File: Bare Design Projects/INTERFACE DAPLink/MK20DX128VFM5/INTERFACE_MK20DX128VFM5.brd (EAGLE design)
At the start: 26 parts, among them CON1 47346-0001, CON2 TC2050-IDC-NL, U2 TLV1117LV33DCYR, U3 IF_MK20DX128VFM5, Y1 CSTCE8M00G55-R0

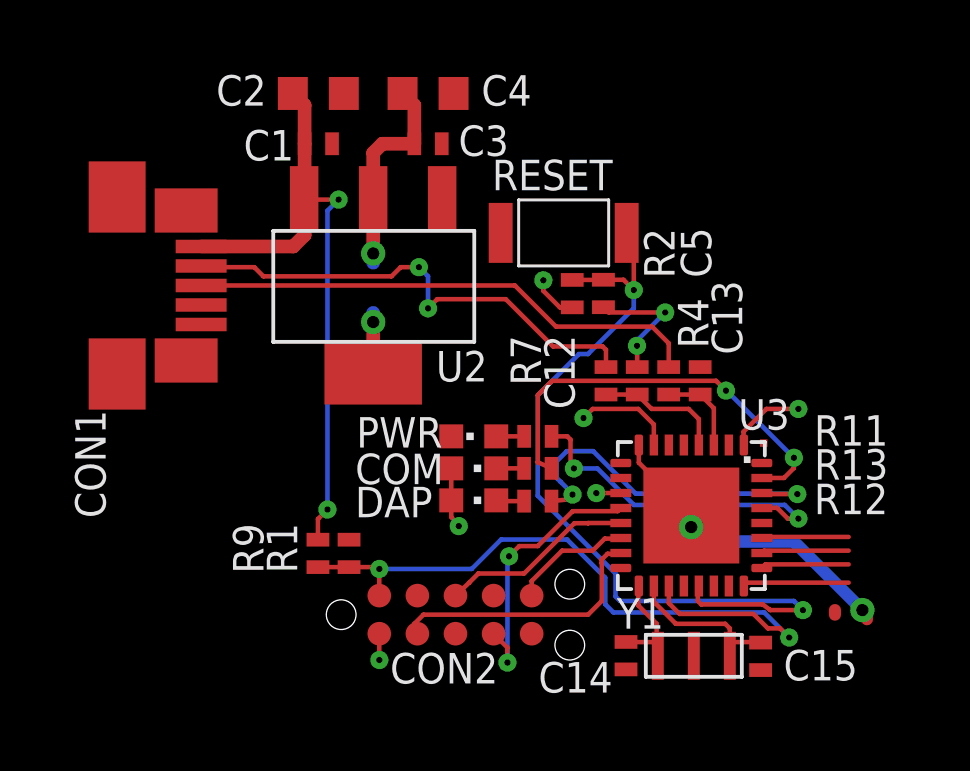
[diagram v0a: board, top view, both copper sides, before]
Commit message: Fixed PDF and name errors
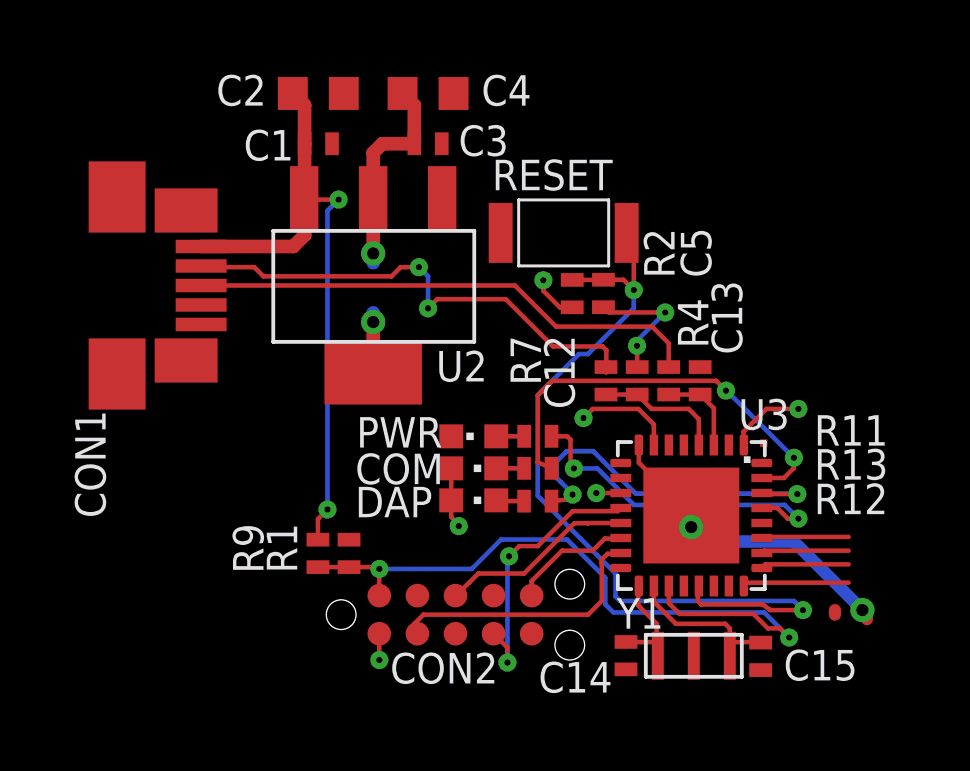
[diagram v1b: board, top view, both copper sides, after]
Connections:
- net DAP_NRESET renamed TGT_NRESET
- net DAP_RX renamed TGT_RX
- net DAP_SWCLK renamed TGT_SWCLK
- net DAP_SWDIO renamed TGT_SWDIO
- net DAP_TX renamed TGT_TX
- net DAP_USB_D+ renamed TGT_USB_D+
- net DAP_USB_D- renamed TGT_USB_D-
- net TCLK renamed IF_SWCLK
- net TDI renamed IF_TDI
- net TDO renamed IF_TDO
- net TMS renamed IF_SWDIO
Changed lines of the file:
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@@
 <wire x1="11.8872" y1="-5.9436" x2="12.0396" y2="-6.096" width="0.4064" layer="1"/>
 <wire x1="12.0396" y1="-6.096" x2="12.0396" y2="-6.2484" width="0.4064" layer="1"/>
+<wire x1="-2.1336" y1="9.6012" x2="-1.7408" y2="11.2776" width="0" layer="19" extent="1-1"/>
+<wire x1="-2.1196" y1="7.7812" x2="-2.1336" y2="9.6012" width="0" layer="19" extent="1-1"/>
+<wire x1="-0.1696" y1="6.6294" x2="-2.1196" y2="7.7812" width="0" layer="19" extent="1-1"/>
+<wire x1="-5.3984" y1="11.2776" x2="-1.7408" y2="11.2776" width="0" layer="19" extent="1-1"/>
+<wire x1="-5.7912" y1="9.6012" x2="-5.3984" y2="11.2776" width="0" layer="19" extent="1-1"/>
+<wire x1="3.25628125" y1="4.1529" x2="-0.1696" y2="6.6294" width="0" layer="19" extent="1-1"/>
+<wire x1="6.479540625" y1="2.156459375" x2="5.52958125" y2="3.977640625" width="0" layer="19" extent="1-1"/>
+<wire x1="4.4349" y1="-0.441459375" x2="4.3815" y2="2.156459375" width="0" layer="19" extent="1-1"/>
+<wire x1="6.17981875" y1="-3.177540625" x2="6.1849" y2="-2.791459375" width="0" layer="19" extent="1-1"/>
+<wire x1="10.9728" y1="-5.9436" x2="11.8872" y2="-5.9436" width="0" layer="19" extent="1-1"/>
+<wire x1="7.4349" y1="-0.441459375" x2="6.1849" y2="-2.791459375" width="0" layer="19" extent="1-1"/>
+<wire x1="8.493759375" y1="-7.942578125" x2="10.9728" y2="-6.096" width="0" layer="19" extent="1-1"/>
+<wire x1="6.2676" y1="-7.4676" x2="8.493759375" y2="-7.942578125" width="0" layer="19" extent="1-1"/>
+<wire x1="4.00811875" y1="-7.91971875" x2="6.2676" y2="-7.4676" width="0" layer="19" extent="1-1"/>
+<wire x1="0.8636" y1="-6.731" x2="4.00811875" y2="-7.91971875" width="0" layer="19" extent="1-1"/>
+<wire x1="-1.6764" y1="-6.731" x2="0.8636" y2="-6.731" width="0" layer="19" extent="1-1"/>
+<wire x1="-5.224778125" y1="-3.596640625" x2="-1.6764" y2="-6.731" width="0" layer="19" extent="1-1"/>
+<wire x1="-1.8168" y1="-0.1524" x2="-5.224778125" y2="-3.596640625" width="0" layer="19" extent="1-1"/>
+<wire x1="-10.154" y1="3.5768" x2="-5.7912" y2="9.6012" width="0" layer="19" extent="1-1"/>
 </signal>
 <signal name="IF_NRESET">
@@
 <wire x1="4.00811875" y1="-7.00531875" x2="4.0132" y2="-7.0104" width="0.1524" layer="1"/>
 <wire x1="4.0132" y1="-7.0104" x2="5.0292" y2="-7.0104" width="0.1524" layer="1"/>
-</signal>
-<signal name="DAP_USB_D-">
-<contactref element="R7" pad="1"/>
-<wire x1="3.3401" y1="2.156459375" x2="3.3401" y2="2.733040625" width="0.1524" layer="1"/>
-<wire x1="3.3401" y1="2.733040625" x2="3.228340625" y2="2.8448" width="0.1524" layer="1"/>
-<wire x1="3.228340625" y1="2.8448" x2="1.5748" y2="2.8448" width="0.1524" layer="1"/>
-<contactref element="CON1" pad="D-"/>
-<wire x1="1.5748" y1="2.8448" x2="0" y2="4.4196" width="0.1524" layer="1"/>
-<wire x1="0" y1="4.4196" x2="-2.286" y2="4.4196" width="0.1524" layer="1"/>
-<wire x1="-2.286" y1="4.4196" x2="-2.5908" y2="4.1148" width="0.1524" layer="1"/>
-<via x="-2.5908" y="4.1148" extent="1-16" drill="0.2032"/>
-<wire x1="-2.5908" y1="4.1148" x2="-2.5908" y2="5.1816" width="0.1524" layer="16"/>
-<wire x1="-2.5908" y1="5.1816" x2="-2.8956" y2="5.4864" width="0.1524" layer="16"/>
-<via x="-2.8956" y="5.4864" extent="1-16" drill="0.2032"/>
-<wire x1="-2.8956" y1="5.4864" x2="-3.5052" y2="5.4864" width="0.1524" layer="1"/>
-<wire x1="-3.5052" y1="5.4864" x2="-3.81" y2="5.1816" width="0.1524" layer="1"/>
-<wire x1="-3.81" y1="5.1816" x2="-8.0772" y2="5.1816" width="0.1524" layer="1"/>
-<wire x1="-8.0772" y1="5.1816" x2="-8.382" y2="5.4864" width="0.1524" layer="1"/>
-<wire x1="-8.382" y1="5.4864" x2="-10.1136" y2="5.4864" width="0.1524" layer="1"/>
-<wire x1="-10.1136" y1="5.4864" x2="-10.154" y2="5.5268" width="0.1524" layer="1"/>
-</signal>
-<signal name="DAP_USB_D+">
-<contactref element="R4" pad="1"/>
-<wire x1="5.43051875" y1="2.156459375" x2="5.43051875" y2="2.95148125" width="0.1524" layer="1"/>
-<wire x1="5.43051875" y1="2.95148125" x2="4.8768" y2="3.5052" width="0.1524" layer="1"/>
-<wire x1="4.8768" y1="3.5052" x2="1.6764" y2="3.5052" width="0.1524" layer="1"/>
-<contactref element="CON1" pad="D+"/>
-<wire x1="-10.154" y1="4.8768" x2="0.3048" y2="4.8768" width="0.1524" layer="1"/>
-<wire x1="0.3048" y1="4.8768" x2="1.6764" y2="3.5052" width="0.1524" layer="1"/>
 </signal>
 <signal name="+3.3V">
@@
 <via x="9.7536" y="0.762" extent="1-16" drill="0.2032"/>
 <wire x1="9.7536" y1="0.762" x2="9.906" y2="0.762" width="0.1524" layer="16"/>
-</signal>
-<signal name="DAP_NRESET">
+<wire x1="-1.56718125" y1="-3.14451875" x2="-4.2164" y2="-6.731" width="0" layer="19" extent="1-16"/>
+<wire x1="-4.4196" y1="1.9812" x2="-1.8168" y2="-1.2192" width="0" layer="19" extent="1-1"/>
+<wire x1="-4.4196" y1="5.6388" x2="-4.4196" y2="3.9624" width="0" layer="19" extent="16-16"/>
+<wire x1="3.037840625" y1="-2.17678125" x2="-1.49098125" y2="-3.14198125" width="0" layer="19" extent="16-16"/>
+<wire x1="4.9349" y1="-0.441459375" x2="3.8349" y2="-2.041459375" width="0" layer="19" extent="1-1"/>
+<wire x1="7.9248" y1="-0.431359375" x2="4.9349" y2="-0.441459375" width="0" layer="19" extent="1-1"/>
+<wire x1="2.21488125" y1="4.14781875" x2="2.8956" y2="0.762" width="0" layer="19" extent="1-1"/>
+</signal>
+<signal name="TGT_NRESET">
 <contactref element="RESET" pad="P$2"/>
 <wire x1="4.0304" y1="6.6294" x2="4.2672" y2="6.3246" width="0.1524" layer="1"/>
@@
 <wire x1="9.906" y1="-5.9436" x2="9.6012" y2="-5.6388" width="0.1524" layer="16"/>
 </signal>
-<signal name="DAP_TX">
+<signal name="TGT_TX">
 <contactref element="U3" pad="24"/>
 <wire x1="7.9349" y1="-5.141459375" x2="8.047159375" y2="-5.0292" width="0.1524" layer="1"/>
@@
 <wire x1="-6.67778125" y1="7.73938125" x2="-6.7196" y2="7.7812" width="0.1524" layer="1"/>
 </signal>
-<signal name="TMS">
+<signal name="IF_SWDIO">
 <contactref element="U3" pad="15"/>
 <contactref element="CON2" pad="2"/>
@@
 <wire x1="3.80981875" y1="-4.066540625" x2="3.8349" y2="-4.041459375" width="0.1524" layer="1"/>
 </signal>
-<signal name="TDO">
+<signal name="IF_TDO">
 <contactref element="U3" pad="14"/>
 <contactref element="CON2" pad="6"/>
@@
 <wire x1="3.815278125" y1="-3.56108125" x2="3.8349" y2="-3.541459375" width="0.1524" layer="1"/>
 </signal>
-<signal name="TDI">
+<signal name="IF_TDI">
 <contactref element="U3" pad="13"/>
 <contactref element="CON2" pad="8"/>
@@
 <wire x1="2.7432" y1="-3.048" x2="2.749740625" y2="-3.041459375" width="0.1524" layer="1"/>
 </signal>
-<signal name="TCLK">
+<signal name="IF_SWCLK">
 <contactref element="U3" pad="12"/>
 <contactref element="CON2" pad="4"/>
@@
 <wire x1="-0.3168" y1="-0.1524" x2="0.612140625" y2="-0.1524" width="0.1524" layer="1"/>
 </signal>
-<signal name="DAP_SWCLK">
+<signal name="TGT_SWCLK">
 <contactref element="U3" pad="26"/>
 <wire x1="8.5349" y1="-4.041459375" x2="8.613959375" y2="-3.9624" width="0.1524" layer="1"/>
 <wire x1="8.613959375" y1="-3.9624" x2="11.43" y2="-3.9624" width="0.1524" layer="1"/>
 </signal>
-<signal name="DAP_SWDIO">
+<signal name="TGT_SWDIO">
 <contactref element="U3" pad="27"/>
 <wire x1="8.5349" y1="-3.541459375" x2="8.571159375" y2="-3.5052" width="0.1524" layer="1"/>
 <wire x1="8.571159375" y1="-3.5052" x2="11.43" y2="-3.5052" width="0.1524" layer="1"/>
 </signal>
-<signal name="DAP_RX">
+<signal name="TGT_RX">
 <contactref element="U3" pad="25"/>
 <wire x1="8.5349" y1="-4.541459375" x2="8.656759375" y2="-4.4196" width="0.1524" layer="1"/>
 <wire x1="8.656759375" y1="-4.4196" x2="11.43" y2="-4.4196" width="0.1524" layer="1"/>
 </signal>
+<signal name="TGT_USB_D+">
+<contactref element="R4" pad="1"/>
+<wire x1="5.43051875" y1="2.95148125" x2="4.8768" y2="3.5052" width="0.1524" layer="1"/>
+<wire x1="4.8768" y1="3.5052" x2="1.6764" y2="3.5052" width="0.1524" layer="1"/>
+<contactref element="CON1" pad="D+"/>
+<wire x1="-10.154" y1="4.8768" x2="0.3048" y2="4.8768" width="0.1524" layer="1"/>
+<wire x1="0.3048" y1="4.8768" x2="1.6764" y2="3.5052" width="0.1524" layer="1"/>
+<wire x1="5.43051875" y1="2.95148125" x2="5.43051875" y2="2.156459375" width="0.1524" layer="1"/>
+</signal>
+<signal name="TGT_USB_D-">
+<contactref element="R7" pad="1"/>
+<wire x1="3.3528" y1="2.720340625" x2="3.228340625" y2="2.8448" width="0.1524" layer="1"/>
+<wire x1="3.228340625" y1="2.8448" x2="1.5748" y2="2.8448" width="0.1524" layer="1"/>
+<contactref element="CON1" pad="D-"/>
+<wire x1="1.5748" y1="2.8448" x2="0" y2="4.4196" width="0.1524" layer="1"/>
+<wire x1="0" y1="4.4196" x2="-2.286" y2="4.4196" width="0.1524" layer="1"/>
+<wire x1="-2.286" y1="4.4196" x2="-2.5908" y2="4.1148" width="0.1524" layer="1"/>
+<via x="-2.5908" y="4.1148" extent="1-16" drill="0.2032"/>
+<wire x1="-2.5908" y1="4.1148" x2="-2.5908" y2="5.1816" width="0.1524" layer="16"/>
+<wire x1="-2.5908" y1="5.1816" x2="-2.8956" y2="5.4864" width="0.1524" layer="16"/>
+<via x="-2.8956" y="5.4864" extent="1-16" drill="0.2032"/>
+<wire x1="-2.8956" y1="5.4864" x2="-3.5052" y2="5.4864" width="0.1524" layer="1"/>
+<wire x1="-3.5052" y1="5.4864" x2="-3.81" y2="5.1816" width="0.1524" layer="1"/>
+<wire x1="-3.81" y1="5.1816" x2="-8.0772" y2="5.1816" width="0.1524" layer="1"/>
+<wire x1="-8.0772" y1="5.1816" x2="-8.382" y2="5.4864" width="0.1524" layer="1"/>
+<wire x1="-8.382" y1="5.4864" x2="-10.1136" y2="5.4864" width="0.1524" layer="1"/>
+<wire x1="-10.1136" y1="5.4864" x2="-10.154" y2="5.5268" width="0.1524" layer="1"/>
+<wire x1="3.3528" y1="2.720340625" x2="3.3528" y2="1.9812" width="0.1524" layer="1"/>
+<wire x1="3.3528" y1="1.9812" x2="3.3401" y2="1.9939" width="0.1524" layer="1"/>
+<wire x1="3.3401" y1="1.9939" x2="3.3401" y2="2.156459375" width="0.1524" layer="1"/>
+</signal>
 </signals>
